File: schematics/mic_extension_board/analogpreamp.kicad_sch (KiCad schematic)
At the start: 45 parts, among them J1 XLR3, J3 Aux In, J6 Input/Output, J7 XLR3, J8 XLR3, U1 TL074, U2 TL072, U4 NE5534

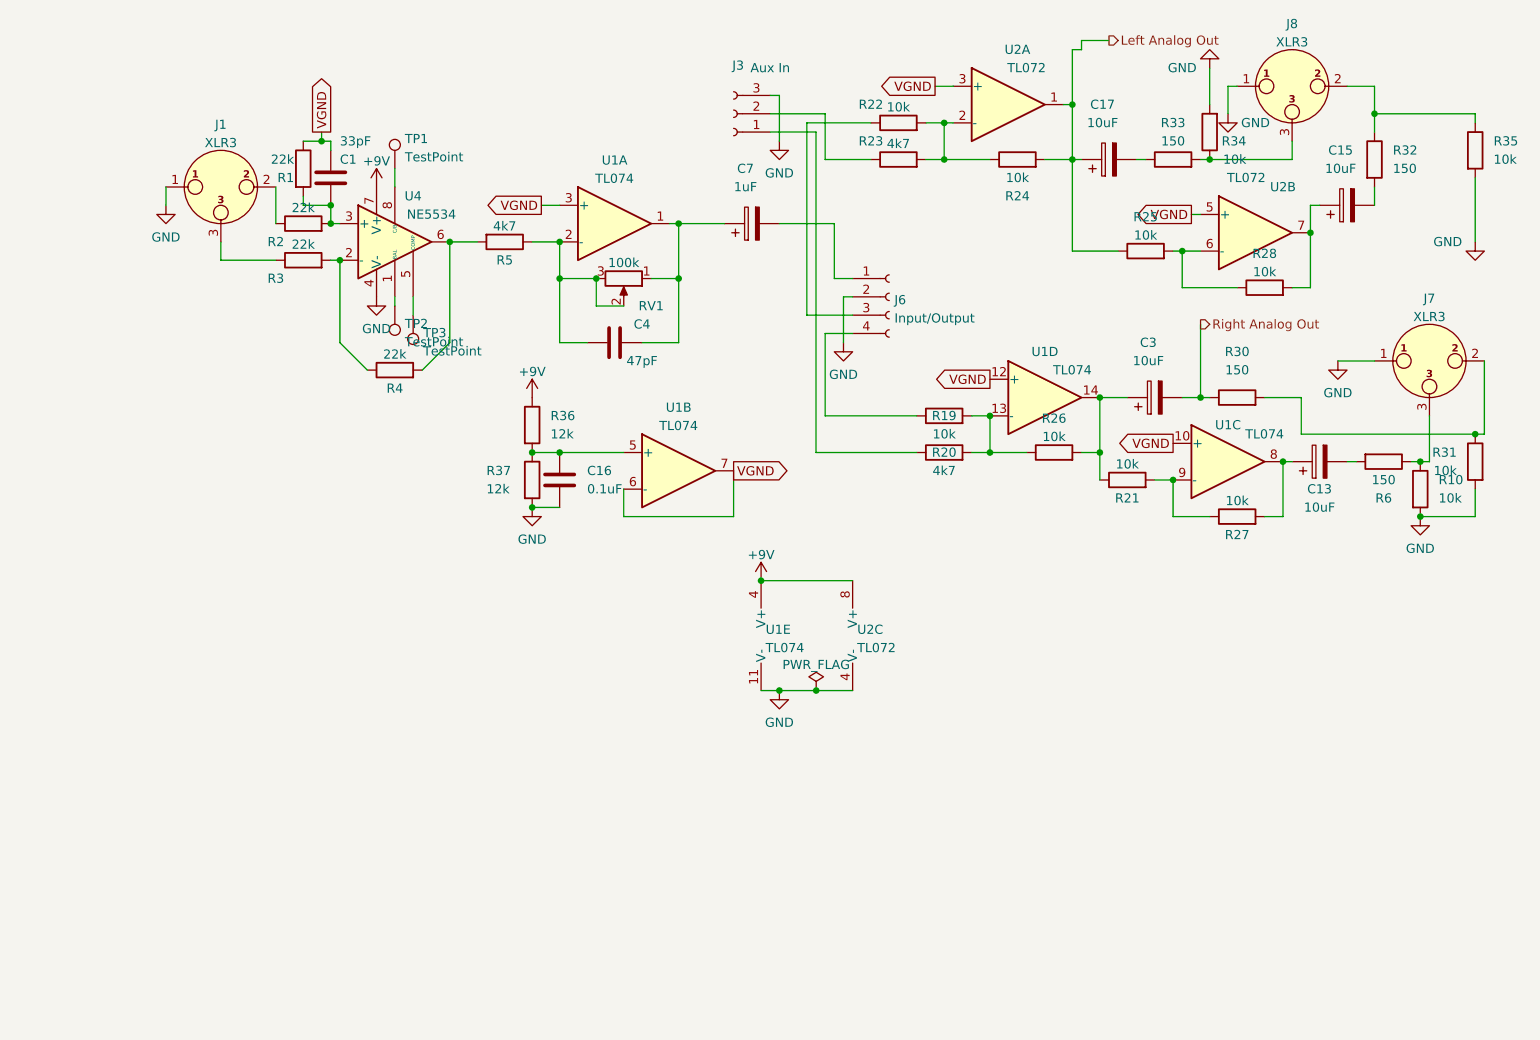
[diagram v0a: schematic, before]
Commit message: more layouting
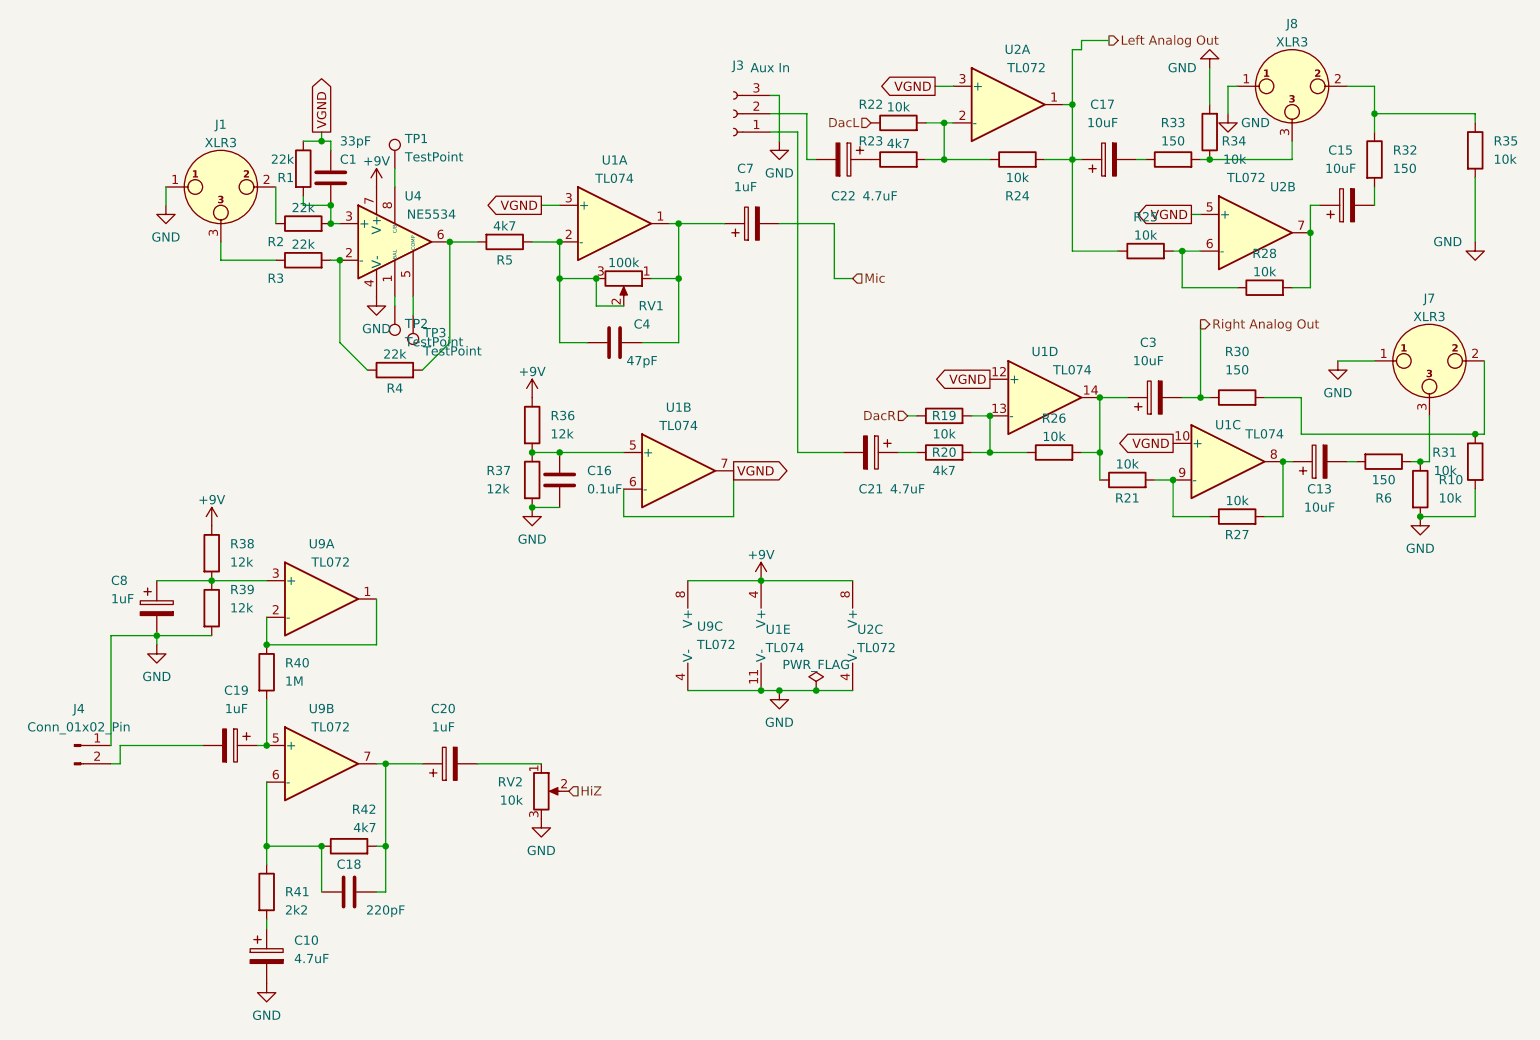
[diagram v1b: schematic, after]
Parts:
- removed J6: Input/Output, Connector_PinHeader_2.54mm:PinHeader_1x04_P2.54mm_Vertical, symbol Connector:Conn_01x04_Female
- added C10, C21, C22: 4.7uF, Capacitor_SMD:CP_Elec_4x4.5, symbol Device:C_Polarized
- added C18: 220pF, Capacitor_SMD:C_0603_1608Metric_Pad1.08x0.95mm_HandSolder, symbol Device:C
- added C19, C20, C8: 1uF, Capacitor_SMD:CP_Elec_4x4.5, symbol Device:C_Polarized
- added J4: Conn_01x02_Pin, Connector_PinHeader_2.54mm:PinHeader_1x02_P2.54mm_Vertical, symbol Connector:Conn_01x02_Pin
- added R38, R39: 12k, Resistor_SMD:R_0603_1608Metric_Pad0.98x0.95mm_HandSolder, symbol Device:R
- added R40: 1M, Resistor_SMD:R_0603_1608Metric_Pad0.98x0.95mm_HandSolder, symbol Device:R
- added R41: 2k2, Resistor_SMD:R_0603_1608Metric_Pad0.98x0.95mm_HandSolder, symbol Device:R
- added R42: 4k7, Resistor_SMD:R_0603_1608Metric_Pad0.98x0.95mm_HandSolder, symbol Device:R
- added RV2: 10k, Connector_PinHeader_2.54mm:PinHeader_1x03_P2.54mm_Vertical, symbol Device:R_Potentiometer
- added U9: TL072, Package_SO:SOIC-8_3.9x4.9mm_P1.27mm, symbol Amplifier_Operational:TL072
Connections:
- net +9V: now also R38.1, U9.8 (V+)
- net GND: now also C10.2, C8.2, J4.1 (Pin_1), R39.2, RV2.3, U9.4 (V-)
- net at R20.1: now also C21.1; no longer J3.1 (Pin_1)
- net Mic: now reaches C7.2
- net DacL: now reaches R22.1
- net DacR: now reaches R19.1
- net at R23.1: now also C22.1; no longer J3.2 (Pin_2)
- new net: C21.2, J3.1 (Pin_1)
- new net: C19.1, R40.2, U9.5 (+)
- new net: C18.1, R41.1, R42.1, U9.6 (-)
- new net: C18.2, C20.1, R42.2, U9.7
- new net: R40.1, U9.1, U9.2 (-)
- new net: C8.1, R38.2, R39.1, U9.3 (+)
- new net: C20.2, RV2.1
- new net: C10.1, R41.2
- new net: C22.2, J3.2 (Pin_2)
- new net: C19.2, J4.2 (Pin_2)
- new net HiZ: RV2.2
